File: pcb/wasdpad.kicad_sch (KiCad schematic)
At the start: 24 parts, among them SW1 SW_Push_45deg, SW2 SW_Push_45deg, SW3 SW_Push_45deg, SW4 SW_Push_45deg, SW5 SW_Push_45deg, SW6 SW_Push_45deg, U1 XIAO-RP2040-DIP

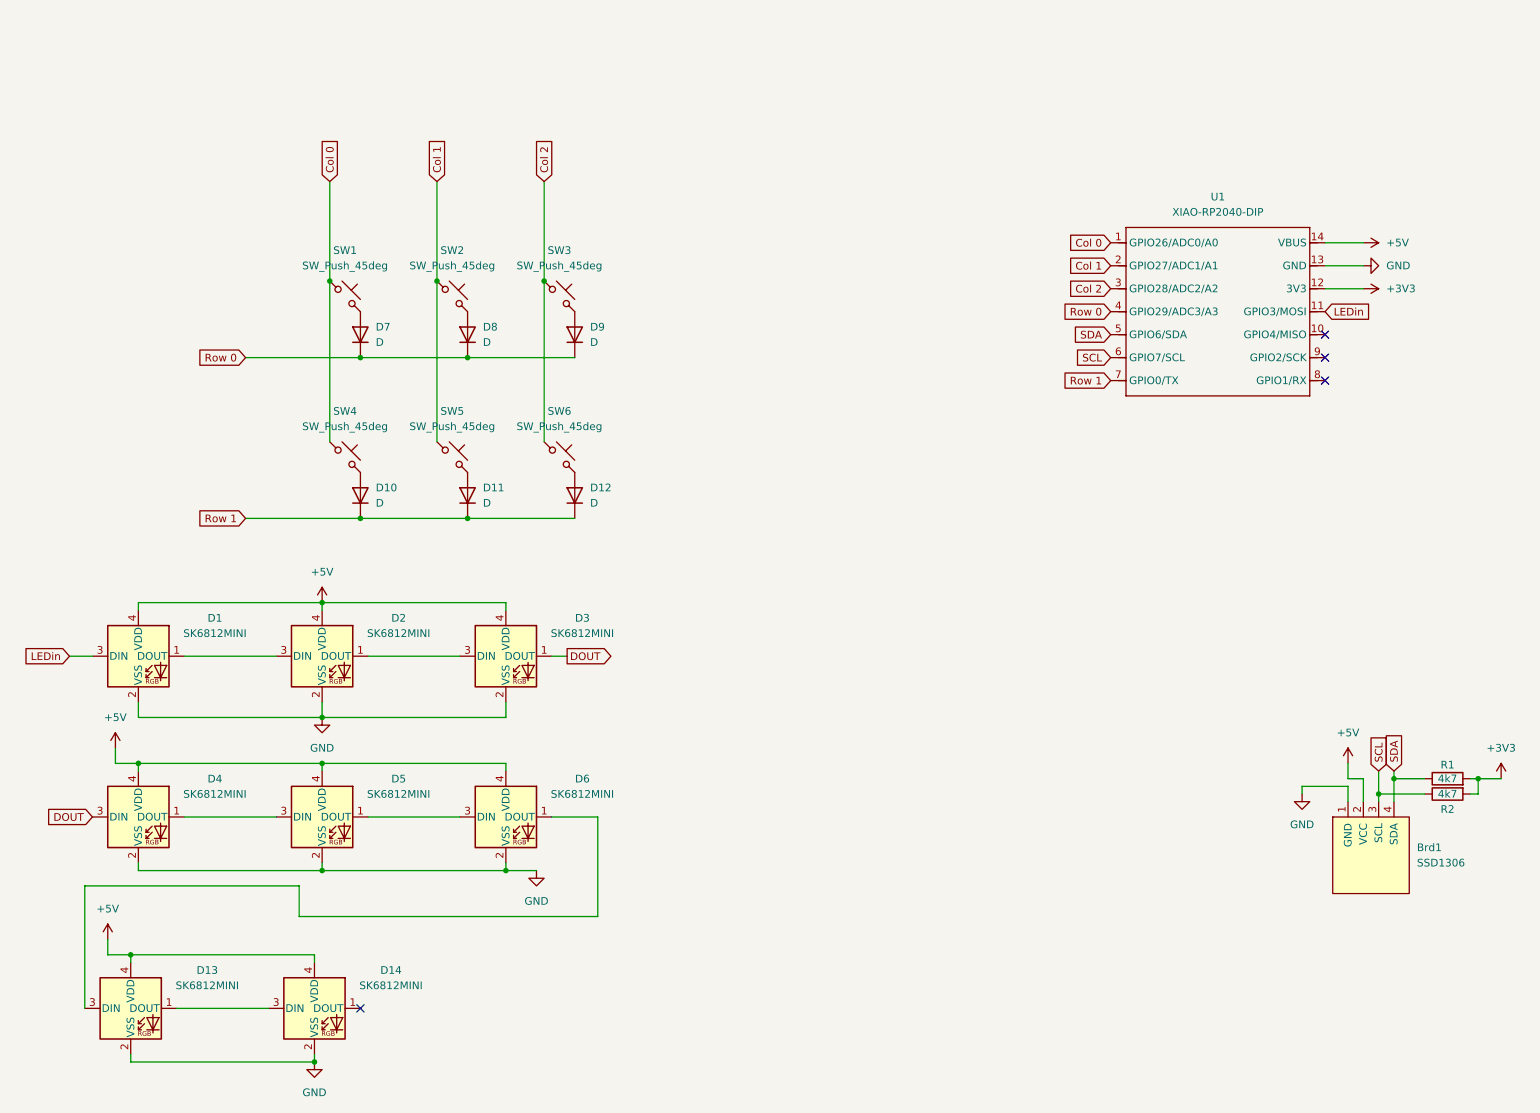
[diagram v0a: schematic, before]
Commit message: add production files
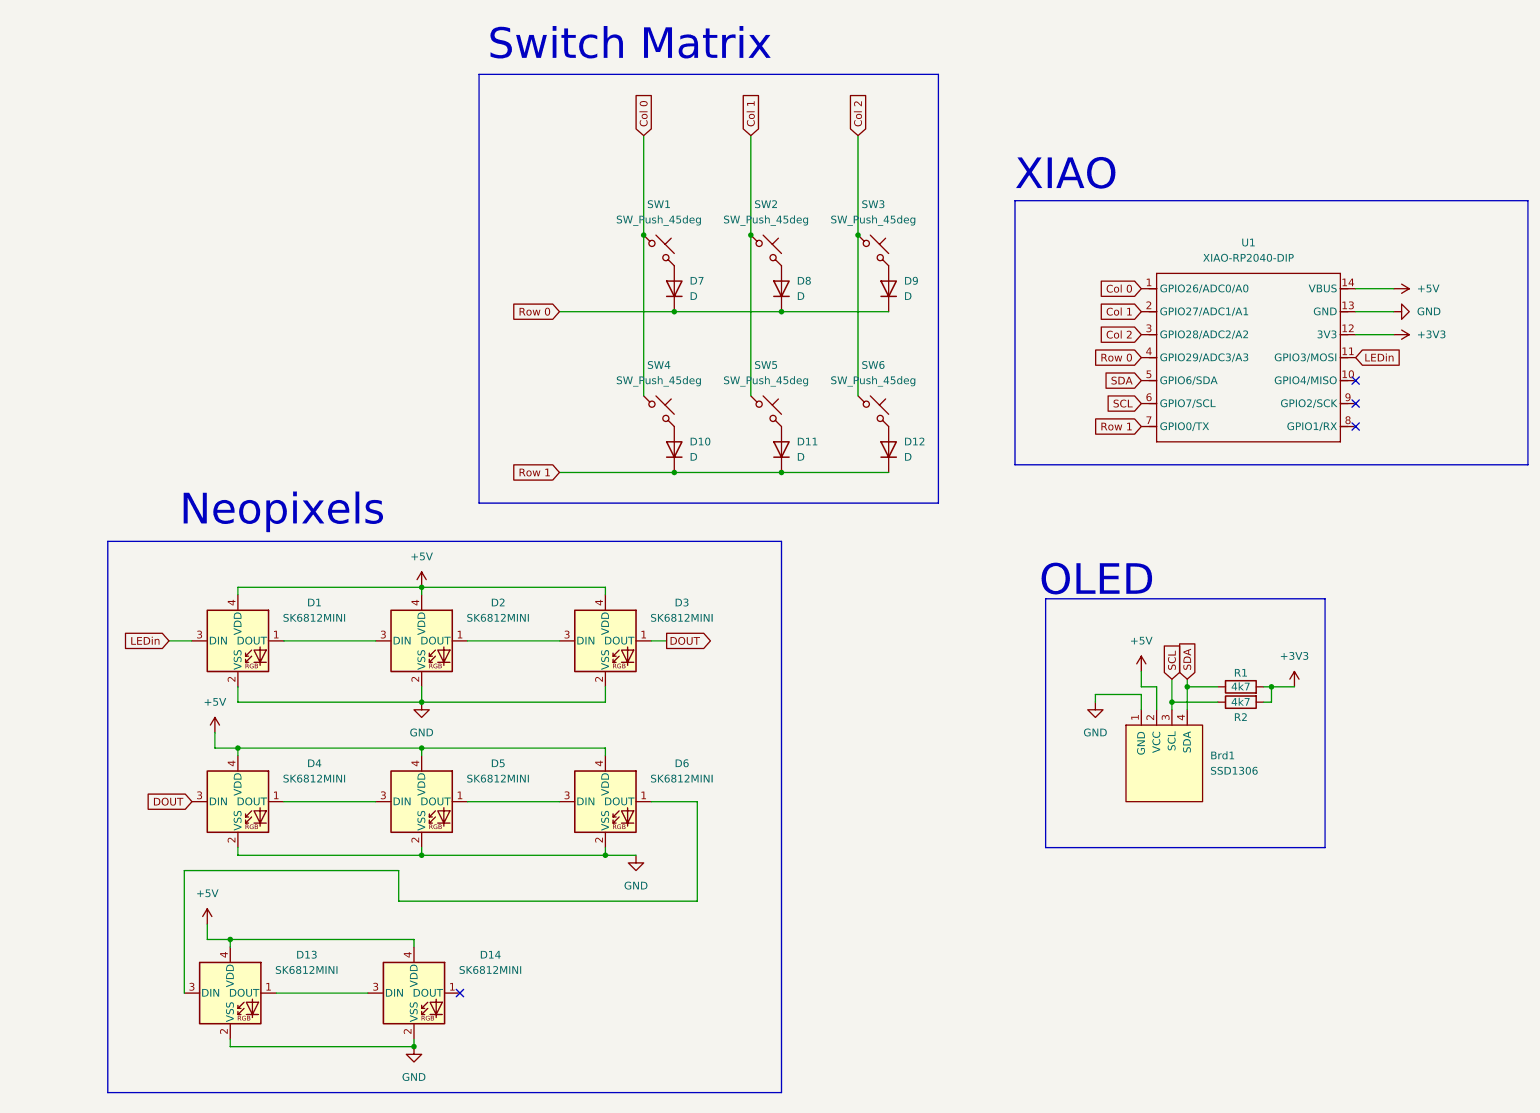
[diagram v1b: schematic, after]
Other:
- note added: "Neopixels"
- note added: "OLED"
- note added: "Switch Matrix"
- note added: "XIAO"
- moved on the sheet: Brd1, D1, D10, D11, D12, D13, D14, D2, D3, D4, D5, D6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
